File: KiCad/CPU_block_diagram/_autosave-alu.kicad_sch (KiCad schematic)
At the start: 8 parts, among them U16 74LS245, U17 74LS283, U18 74LS283, U19 74LS86, U20 74LS86, U21 74LS02, U22 74LS08

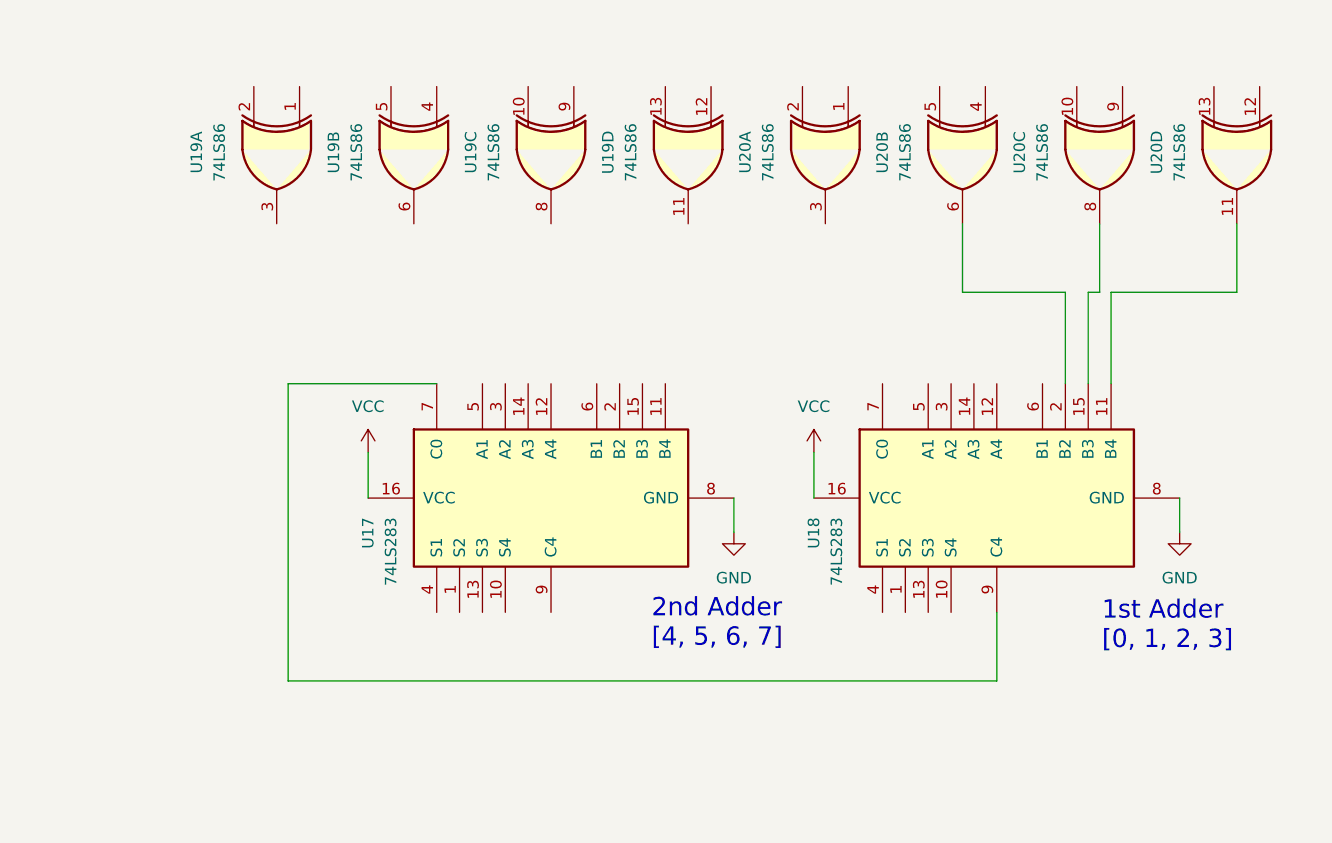
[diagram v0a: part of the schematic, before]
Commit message: vault backup: 2026-01-15 03:11:46
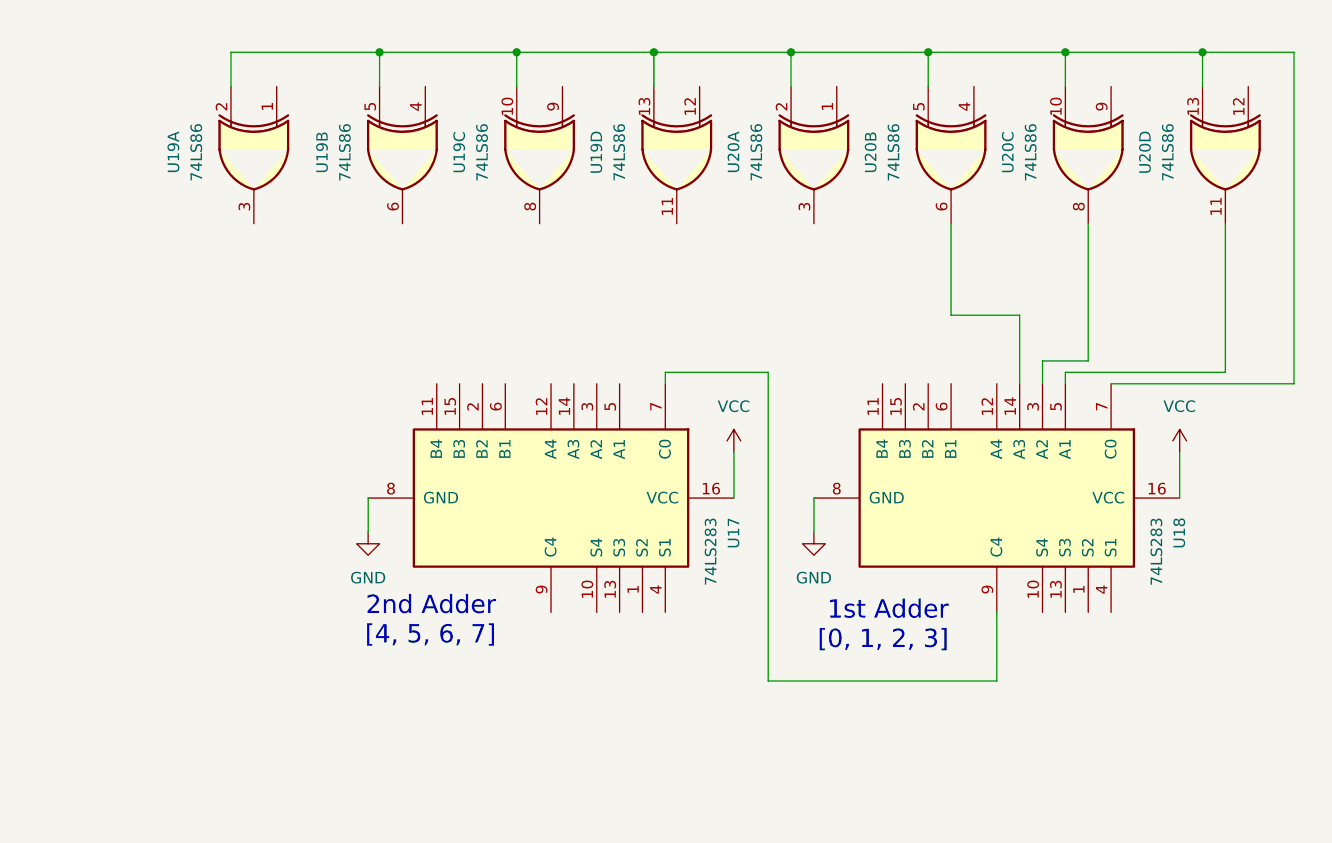
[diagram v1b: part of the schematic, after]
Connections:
- net at U20.5: now also U18.7 (C0), U19.10, U19.13, U19.2, U19.5, U20.10, U20.13, U20.2
- net at U20.6: now also U18.14 (A3); no longer U18.2 (B2)
- net at U18.11 (B4): no longer U20.11
- net at U18.15 (B3): no longer U20.8
- net at U18.3 (A2): now also U20.8
- net at U18.5 (A1): now also U20.11
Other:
- moved on the sheet: U17, U18, U19A, U19B, U19C, U19D, U20A, U20B, U20C, U20D
